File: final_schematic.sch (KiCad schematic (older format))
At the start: 59 parts, among them J1 USB_B_Micro, J2 Conn_Coaxial, J3 Conn_01x04_Male, U1 BQ27441-G1, U2 BQ24075, U3 MTK3339, U4 XC6220B331MR, U5 XC6220B331MR, U6 STM32L476VGTx, U7 RFM95W-868S2, U8 UG-2856KLBAG01_4WSPI, U9 BNO055, X1 SMA_EDGE_UFL

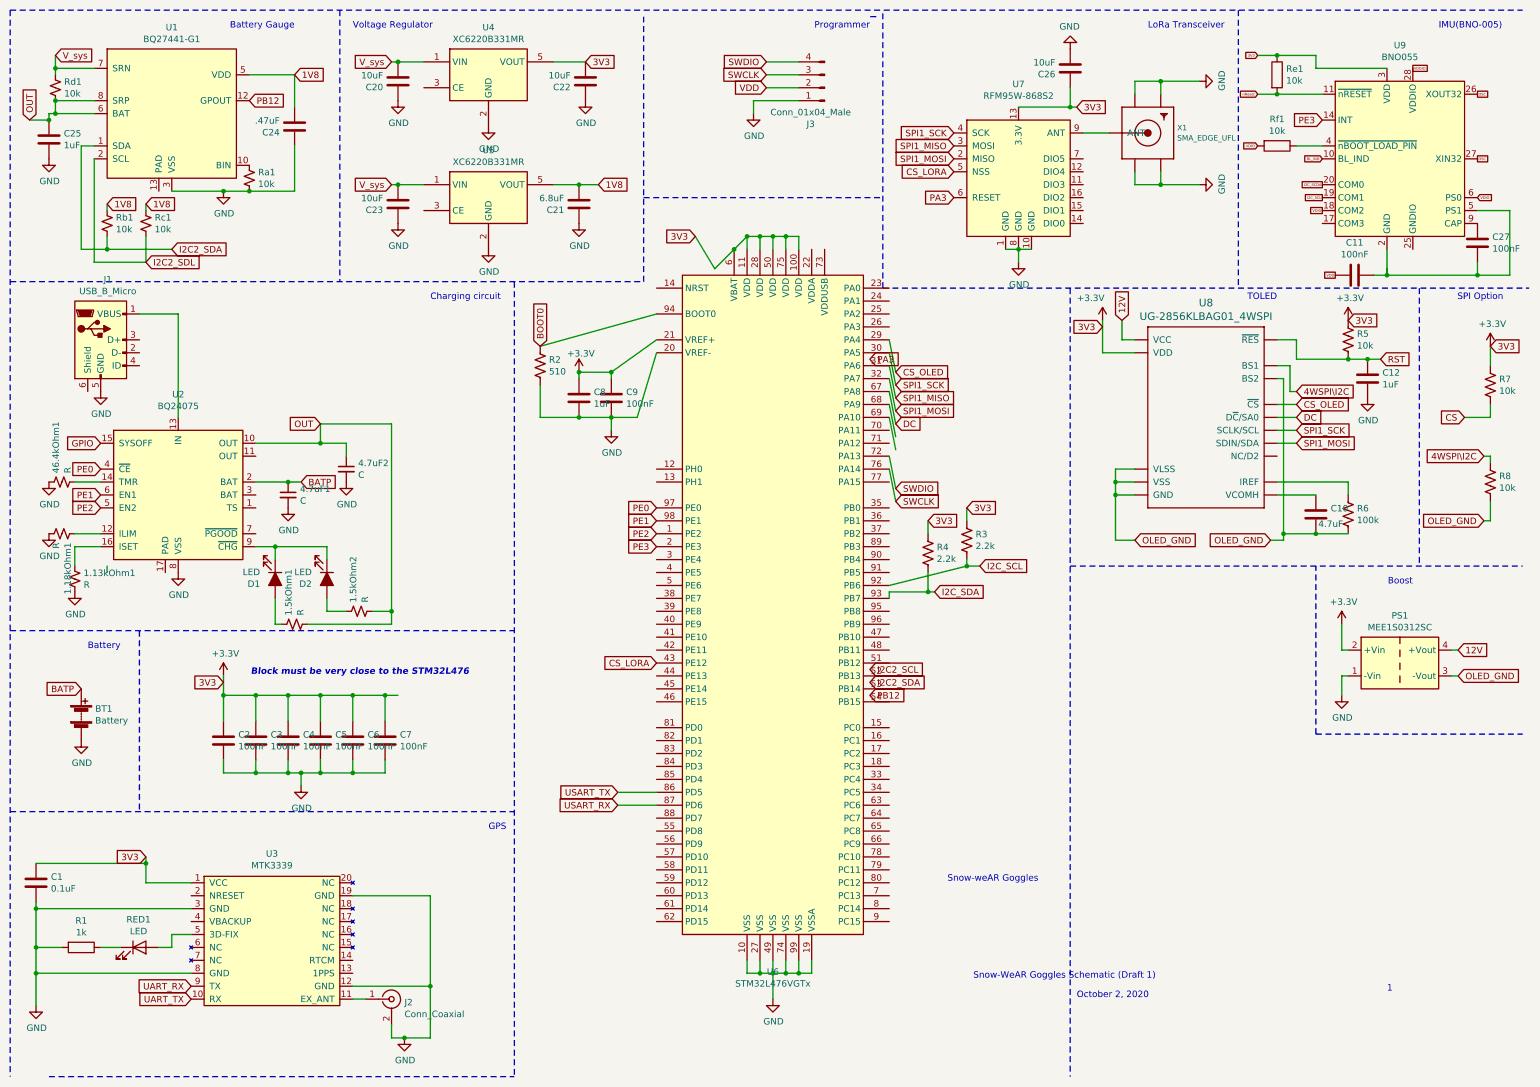
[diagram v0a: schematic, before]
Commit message: made original draft look neater. Now I need to actually do work
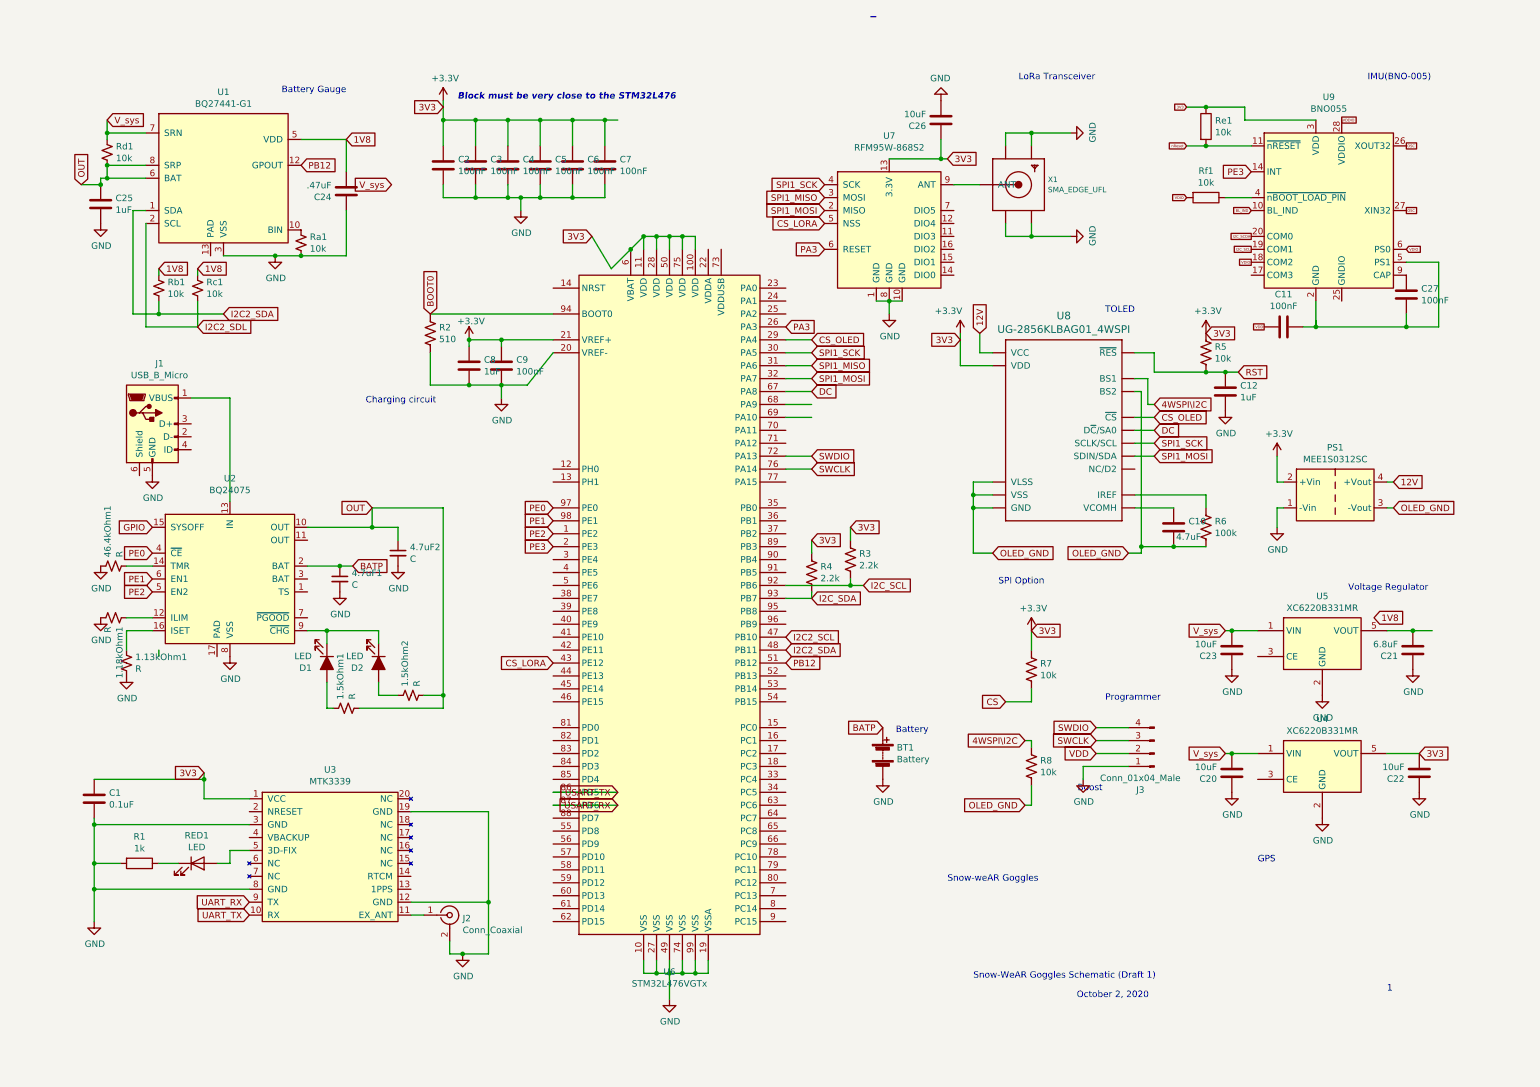
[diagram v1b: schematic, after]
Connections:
- wire segments 242 -> 240
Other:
- moved on the sheet: 1.13kOhm1, 1.18kOhm1, 1.5kOhm1, 1.5kOhm2, 4.7uF1, 4.7uF2, 46.4kOhm1, BT1, C1, C10, C11, C12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
